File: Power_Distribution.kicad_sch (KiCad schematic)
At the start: 0 parts

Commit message: Updated power distribution design
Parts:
- added C1: 10uF, UTSVT_Passive:C_2220_5750Metric, symbol Device:C
- added C2, C3: 10uF, Capacitor_SMD:C_0805_2012Metric, symbol Device:C
- added C4: 10uF, symbol Device:C
- added C5: C, symbol Device:C
- added D2: PowerLED, LED_SMD:LED_0805_2012Metric, symbol Device:LED
- added D3: SD12_SOD323, Diode_SMD:D_SOD-323, symbol Diode:SD12_SOD323
- added D4: D_Zener, symbol Device:D_Zener
- added FB1: 5VFB, Inductor_SMD:L_0805_2012Metric, symbol Device:FerriteBead_Small
- added Q1: Q_PMOS_GSD, Package_TO_SOT_SMD:SuperSOT-3, symbol Device:Q_PMOS_GSD
- added Q2, Q3: NPN, symbol Simulation_SPICE:NPN
- added R1, R2, R4: 1k, Resistor_SMD:R_0805_2012Metric, symbol Device:R
- added R3: 100, Resistor_SMD:R_0805_2012Metric, symbol Device:R
- added TP1: +12V_TP, TestPoint:TestPoint_Keystone_5005-5009_Compact, symbol Connector:TestPoint
- added TP2: GNDPWR_TP, TestPoint:TestPoint_Keystone_5005-5009_Compact, symbol Connector:TestPoint
- added TP3: +5V_TP, TestPoint:TestPoint_Keystone_5005-5009_Compact, symbol Connector:TestPoint
- added TP4: GND_TP, TestPoint:TestPoint_Keystone_5005-5009_Compact, symbol Connector:TestPoint
- added U2: RI3-1205S, UTSVT_ICs:RI3_DC_Converter, symbol utsvt-power-regulators:RI3-1205S
- added U3: LD1117-3.3_SOT223, Package_TO_SOT_SMD:SOT-223-3_TabPin2, symbol Regulator_Linear:LD1117S33TR_SOT223
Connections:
- new net: Q1.1 (G), R2.1
- new net: C4.1, Q2.2 (B), R3.2
- new net: C5.1, D4.1 (K), Q3.2 (B), R4.2
- new net: Q2.3 (E), Q3.1 (C), R4.1
- new net: D2.2 (A), R1.2
- new net: C1.1, Q1.3 (D), TP1.1, U2.2 (+Vin)
- new net +3.3V: C3.1, R1.1, U3.2 (VO)
- new net +5V: Q2.1 (C), R3.1, TP3.1, U2.4 (+Vout)
- new net 12V_Ext: FB1.2
- new net 5V_Clean: C2.1, Q3.3 (E), U3.3 (VI)
- new net 5V_Ferrite: D3.2 (A2), FB1.1, Q1.2 (S)
- new net GND: C2.2, C3.2, C4.2, C5.2, D2.1 (K), D4.2 (A), TP4.1, U2.3 (-Vout), U3.1 (GND)
- new net GNDPWR: C1.2, D3.1 (A1), R2.2, TP2.1, U2.1 (-Vin)
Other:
- note added: "+5V (unisolated) to +5V (isolated)"
- note added: "+5V is already isolated so no need to isolate +3.3V Check datasheet for DCDC to simulate ripple might be around 100kHz 50ish mV also simulate 60Hz Simulate with just LDO, capacitance multiplier and LDO, regulator and LDO, and all three and analyze how the frequency response changes"
- note added: "5V to 3.3V"
- note added: "D"
- note added: "G"
- note added: "ISOLATED"
- note added: "Isolated DC-DC Converter for +5V power to an isolated +5V. The input gnd (Power GND) is different from the output gnd (Local GND)"
- note added: "Local GND (Internal)"
- note added: "Power GND (External)"
- note added: "Replace ferrite bead"
- note added: "S"
- note added: "Vin protection"

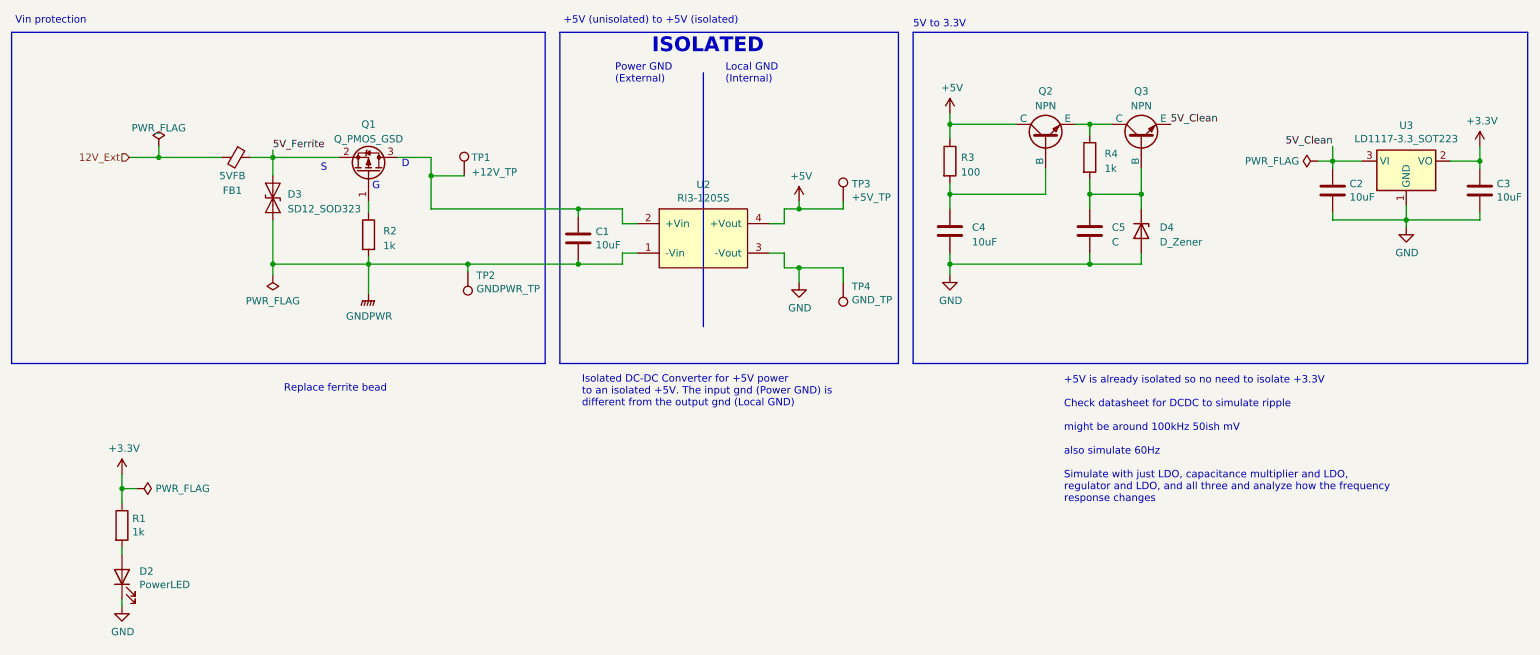
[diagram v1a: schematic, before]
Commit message: Updated power filtering
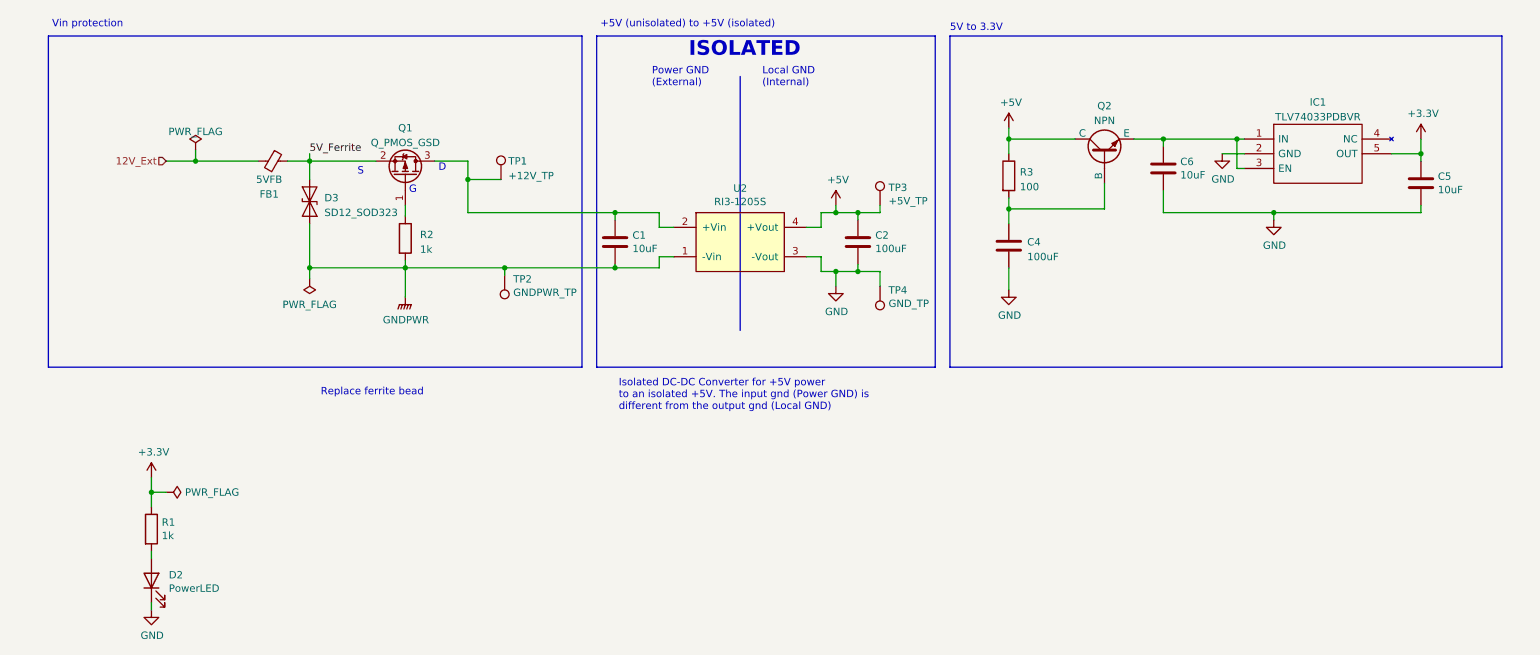
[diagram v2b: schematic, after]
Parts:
- removed C3: 10uF, Capacitor_SMD:C_0805_2012Metric, symbol Device:C
- removed D4: D_Zener, symbol Device:D_Zener
- removed Q3: NPN, symbol Simulation_SPICE:NPN
- removed R4: 1k, Resistor_SMD:R_0805_2012Metric, symbol Device:R
- removed U3: LD1117-3.3_SOT223, Package_TO_SOT_SMD:SOT-223-3_TabPin2, symbol Regulator_Linear:LD1117S33TR_SOT223
- added C6: 10uF, Capacitor_SMD:C_0805_2012Metric, symbol Device:C
- added IC1: TLV74033PDBVR, SOT95P280X145-5N, symbol UTSVT_LeaderSOM:TLV74033PDBVR
- C2: value 10uF -> 100uF; footprint Capacitor_SMD:C_0805_2012Metric -> UTSVT_Passive:C_2220_5750Metric; Mouser Part Number 581-0805YC106KAT2A -> 581-22201C106KAT2A; P/N 0805YC106KAT2A -> 22201C106KAT2A
- C4: value 10uF -> 100uF
- C5: value C -> 10uF; footprint (none) -> Capacitor_SMD:C_0805_2012Metric; Mouser Part Number (none) -> 581-0805YC106KAT2A; P/N (none) -> 0805YC106KAT2A
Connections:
- net 5V_Clean is gone; now on net +5V: C2.1
- net +3.3V: now also C5.1, IC1.5 (OUT)
- net GND: now also C6.2, IC1.2 (GND)
- net at Q2.3 (E): now also C6.1, IC1.1 (IN), IC1.3 (EN)
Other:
- note removed: "+5V is already isolated so no need to isolate +3.3V Check datasheet for DCDC to simulate ripple might be around 100kHz 50ish mV also simulate 60Hz Simulate with just LDO, capacitance multiplier and LDO, regulator and LDO, and all three and analyze how the frequency response changes"
- moved on the sheet: C1, C4, D2, D3, FB1, Q1, Q2, R1, R2, R3, TP1, TP2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

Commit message: Finished power distribution
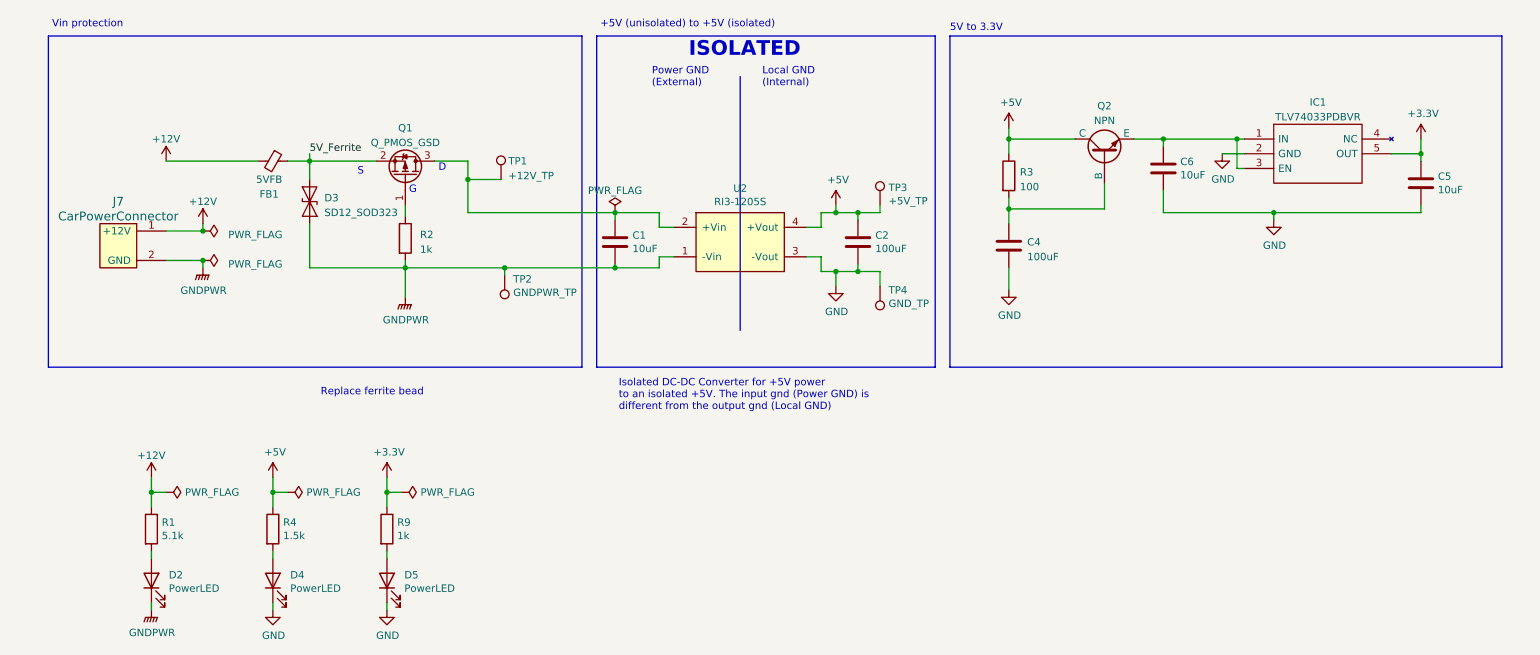
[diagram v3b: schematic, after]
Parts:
- added D4, D5: PowerLED, LED_SMD:LED_0805_2012Metric, symbol Device:LED
- added J7: CarPowerConnector, symbol utsvt-connectors:CarPowerConnector
- added R4: 1.5k, Resistor_SMD:R_0805_2012Metric, symbol Device:R
- added R9: 1k, Resistor_SMD:R_0805_2012Metric, symbol Device:R
- R1: value 1k -> 5.1k
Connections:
- net +3.3V: now also R9.1; no longer R1.1
- net +5V: now also R4.1
- net GND: now also D4.1 (K), D5.1 (K); no longer D2.1 (K)
- net GNDPWR: now also D2.1 (K), J7.2 (GND)
- net 12V_Ext renamed +12V
- net +12V: now also R1.1, J7.1 (+12V)
- new net: D4.2 (A), R4.2
- new net: D5.2 (A), R9.2

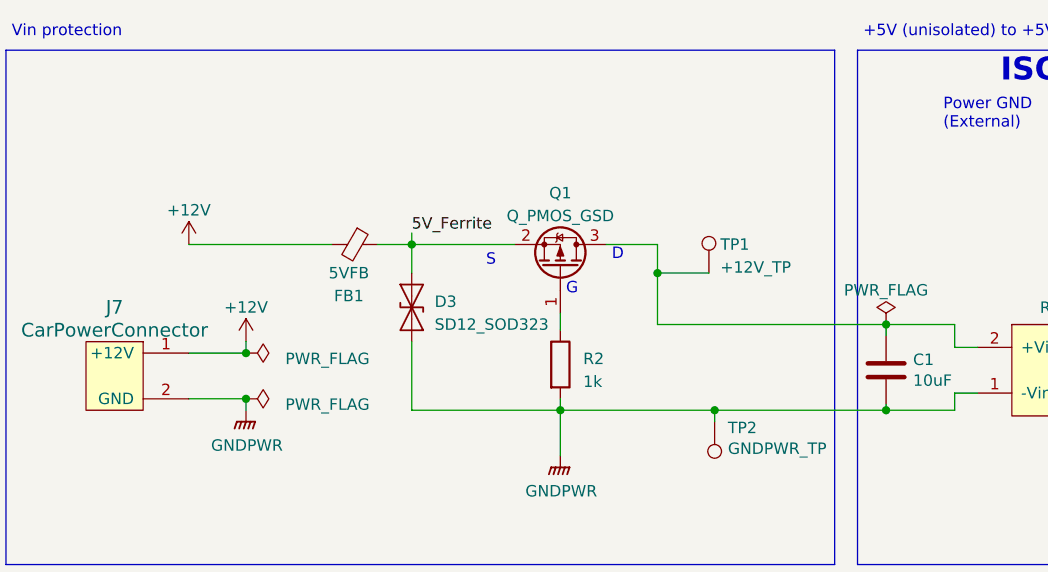
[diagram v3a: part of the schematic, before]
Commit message: Updated CAN circuitry and used new power protection PMOS
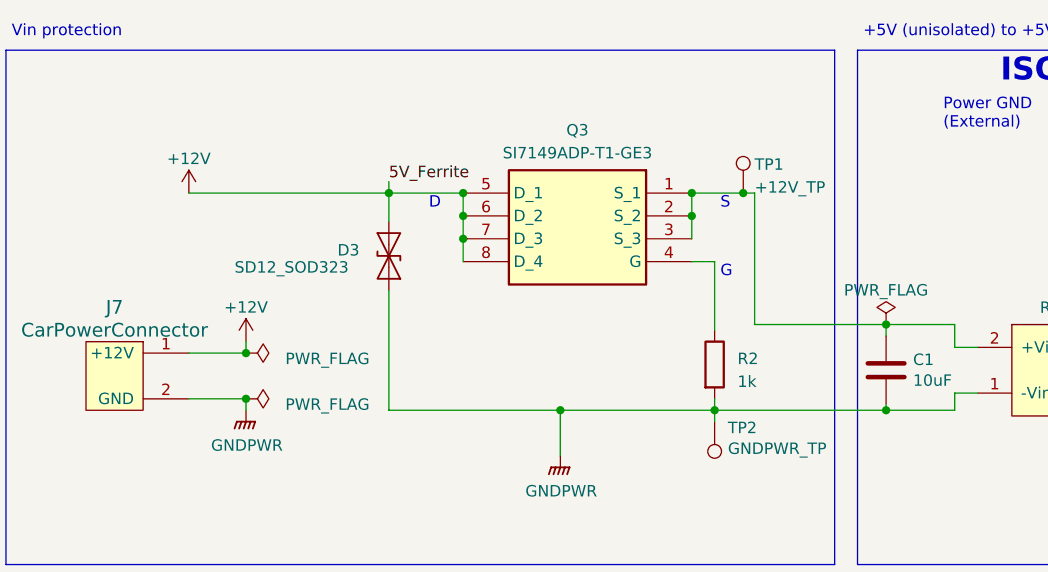
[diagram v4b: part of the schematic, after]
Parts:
- removed FB1: 5VFB, Inductor_SMD:L_0805_2012Metric, symbol Device:FerriteBead_Small
- removed Q1: Q_PMOS_GSD, Package_TO_SOT_SMD:SuperSOT-3, symbol Device:Q_PMOS_GSD
- added Q3: SI7149ADP-T1-GE3, POWERPAKSO-8, symbol UTSVT_LeaderSOM:SI7149ADP-T1-GE3
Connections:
- net 5V_Ferrite is gone; now on net +12V: D3.2 (A2)
- net +12V: now also Q3.5 (D_1), Q3.6 (D_2), Q3.7 (D_3), Q3.8 (D_4)
- net at R2.1: now also Q3.4 (G)
- net at C1.1, TP1.1, U2.2 (+Vin): now also Q3.1 (S_1), Q3.2 (S_2), Q3.3 (S_3)
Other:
- moved on the sheet: D3, R2, TP1
